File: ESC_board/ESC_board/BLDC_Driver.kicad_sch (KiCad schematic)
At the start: 55 parts, among them IC2 DRV8320, J5 Conn_01x03, Q1 TPH2R306NH1,LQ, Q2 TPH2R306NH1,LQ, Q3 TPH2R306NH1,LQ, Q4 TPH2R306NH1,LQ, Q5 TPH2R306NH1,LQ, Q6 TPH2R306NH1,LQ, U2 INA240A1D, U3 INA240A1D, U4 INA240A1D

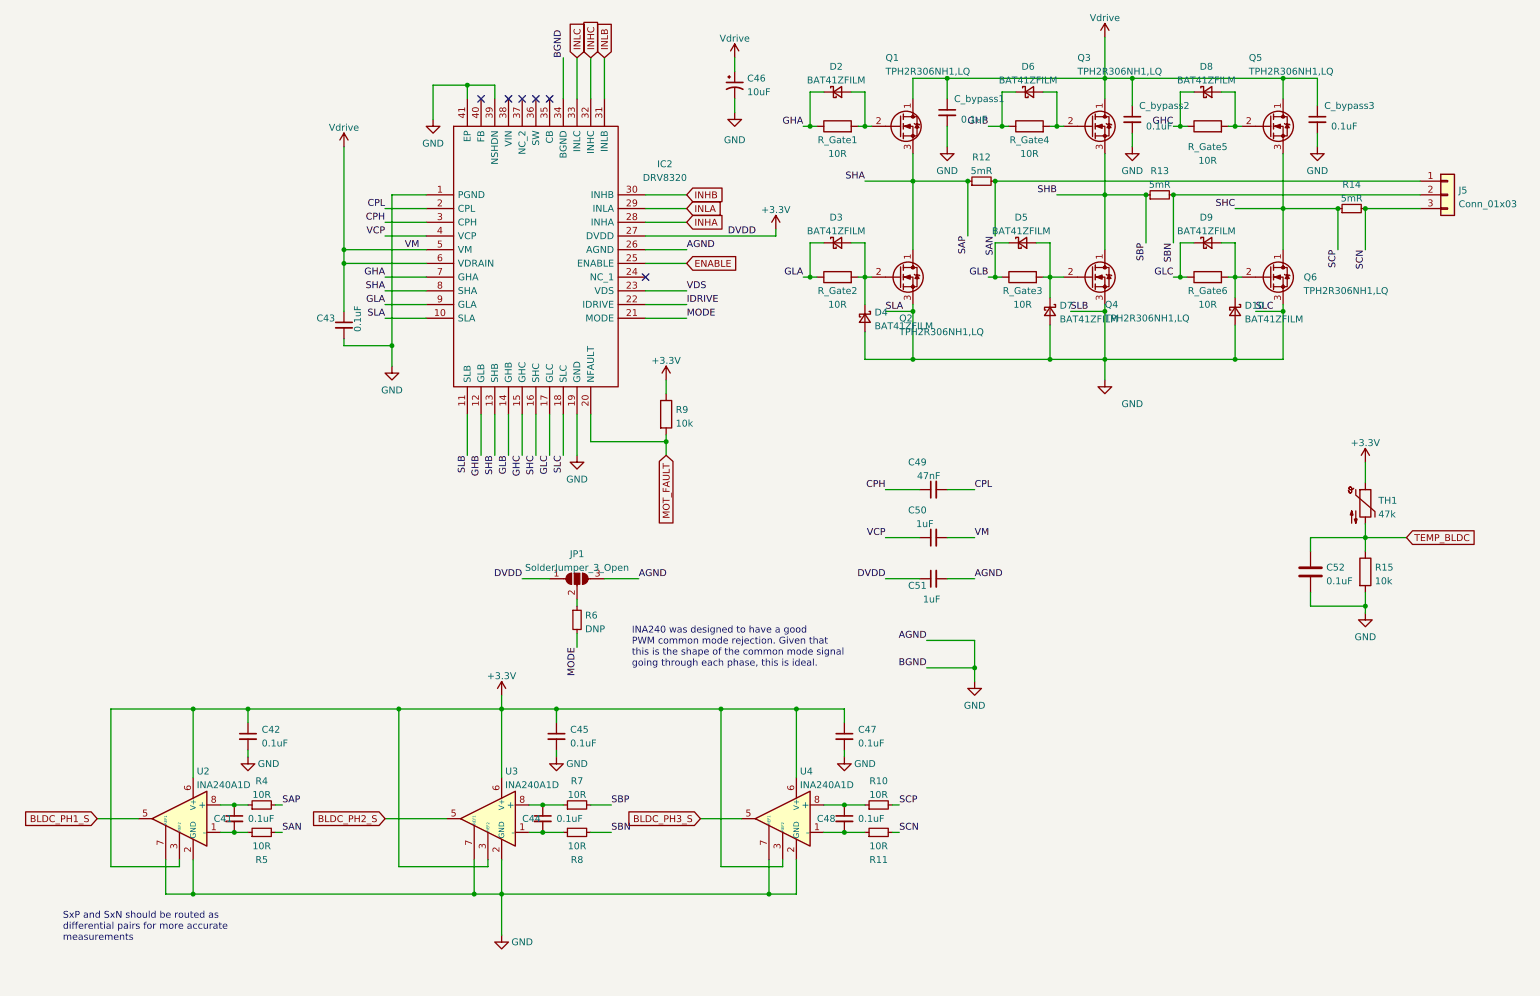
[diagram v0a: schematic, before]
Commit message: Rev 1.2 - Ready for review
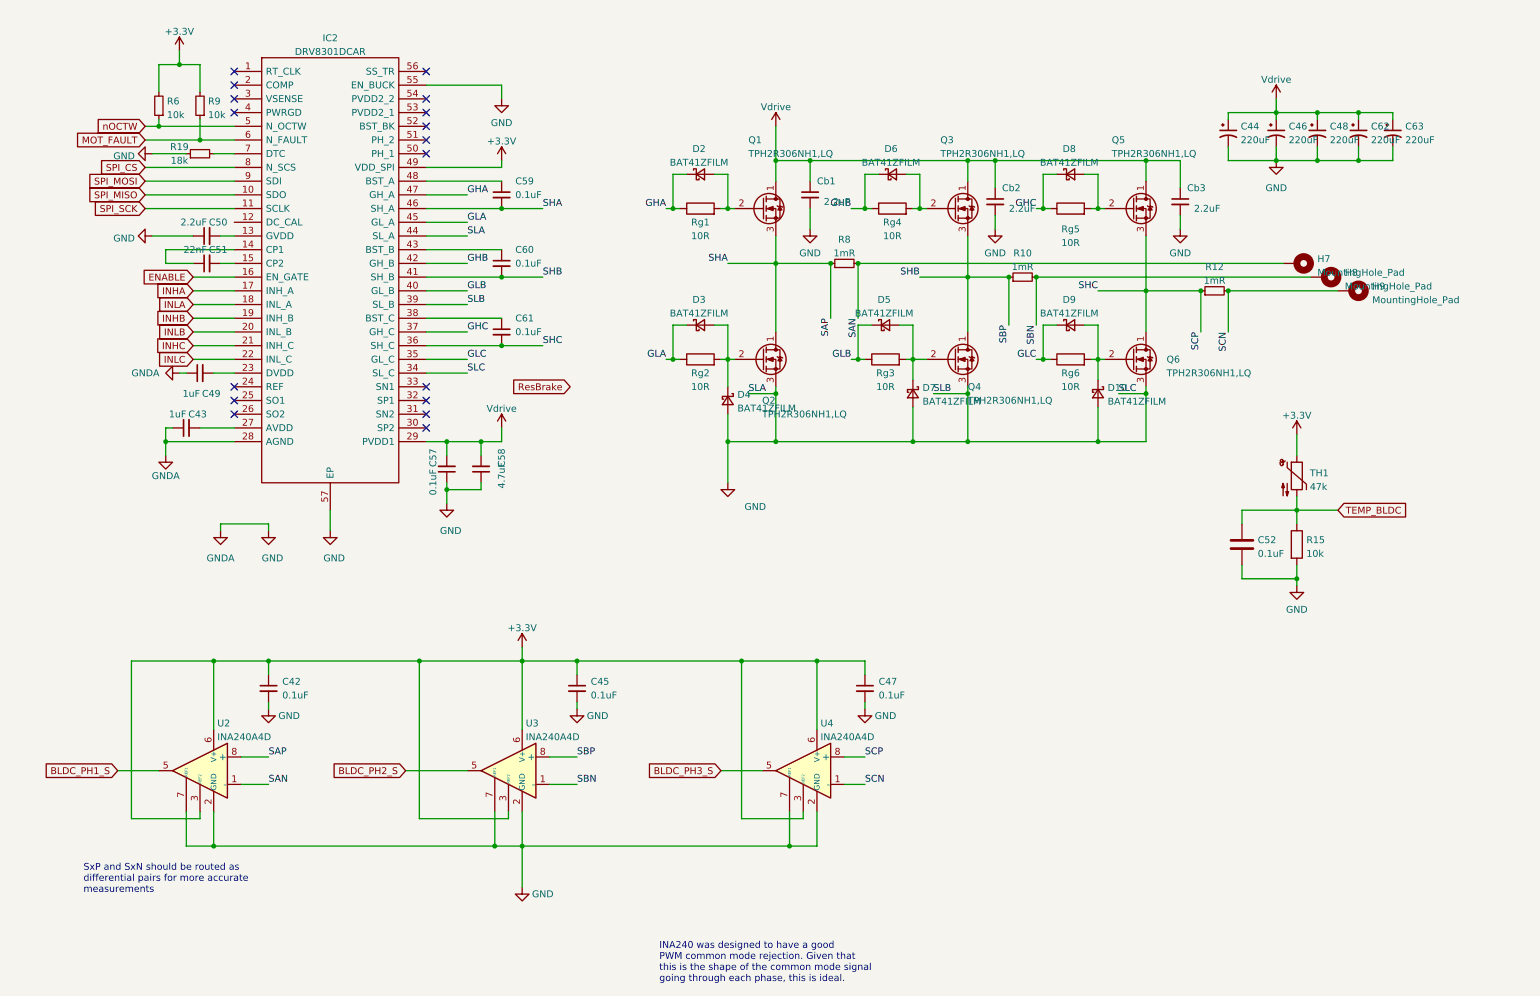
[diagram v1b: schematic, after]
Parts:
- removed C41, C44, C48: 0.1uF, Capacitor_SMD:C_0402_1005Metric_Pad0.74x0.62mm_HandSolder, symbol Device:C_Small
- removed IC2: DRV8320, Package_DFN_QFN:Texas_S-PVQFN-N40_EP4.15x4.15mm_ThermalVias, symbol custom_lib:DRV8320RHRHAT
- removed J5: Conn_01x03, TerminalBlock:TerminalBlock_Altech_AK300-3_P5.00mm, symbol Connector_Generic:Conn_01x03
- removed JP1: SolderJumper_3_Open, Jumper:SolderJumper-3_P2.0mm_Open_TrianglePad1.0x1.5mm_NumberLabels, symbol Jumper:SolderJumper_3_Open
- removed R11, R4, R5, R7: 10R, Resistor_SMD:R_0402_1005Metric_Pad0.72x0.64mm_HandSolder, symbol Device:R_Small
- removed R13, R14: 5mR, Resistor_SMD:R_2010_5025Metric_Pad1.40x2.65mm_HandSolder, symbol Device:R_Small
- removed R9: 10k, Capacitor_SMD:C_0402_1005Metric_Pad0.74x0.62mm_HandSolder, symbol Device:R
- added C44, C48, C62, C63: 220uF, Capacitor_SMD:CP_Elec_5x5.8, symbol Device:C_Polarized_Small_US
- added C57: 0.1uF, Capacitor_SMD:C_0805_2012Metric_Pad1.18x1.45mm_HandSolder, symbol Device:C_Small
- added C58: 4.7uF, Capacitor_SMD:C_0805_2012Metric_Pad1.18x1.45mm_HandSolder, symbol Device:C_Small
- added C59, C60, C61: 0.1uF, Capacitor_SMD:C_0402_1005Metric_Pad0.74x0.62mm_HandSolder, symbol Device:C_Small
- added H7, H8, H9: MountingHole_Pad, Connector_Wire:SolderWire-1.5sqmm_1x01_D1.7mm_OD3.9mm, symbol Mechanical:MountingHole_Pad
- added IC2: DRV8301DCAR, Package_SO:HTSSOP-56-1EP_6.1x14mm_P0.5mm_EP3.61x6.35mm, symbol custom_lib:DRV8301DCAR
- added R19: 18k, Resistor_SMD:R_0402_1005Metric_Pad0.72x0.64mm_HandSolder, symbol Device:R_Small
- added R9: 10k, Resistor_SMD:R_0402_1005Metric_Pad0.72x0.64mm_HandSolder, symbol Device:R_Small
- C43: value 0.1uF -> 1uF
- C46: value 10uF -> 220uF
- C49: value 47nF -> 1uF; footprint Capacitor_SMD:C_0603_1608Metric_Pad1.08x0.95mm_HandSolder -> Capacitor_SMD:C_0402_1005Metric_Pad0.74x0.62mm_HandSolder; Voltage 48V -> 60V
- C50: value 1uF -> 2.2uF; footprint Capacitor_SMD:C_0805_2012Metric_Pad1.18x1.45mm_HandSolder -> Capacitor_SMD:C_0402_1005Metric_Pad0.74x0.62mm_HandSolder; Voltage 16V -> 60V
- C51: value 1uF -> 22nF; footprint Capacitor_SMD:C_0805_2012Metric_Pad1.18x1.45mm_HandSolder -> Capacitor_SMD:C_0603_1608Metric_Pad1.08x0.95mm_HandSolder; Voltage 6.3V -> 100V
- Cb1: renamed from C_bypass1; value 0.1uF -> 2.2uF
- Cb2: renamed from C_bypass2; value 0.1uF -> 2.2uF
- Cb3: renamed from C_bypass3; value 0.1uF -> 2.2uF
- R10, R8: value 10R -> 1mR; footprint Resistor_SMD:R_0402_1005Metric_Pad0.72x0.64mm_HandSolder -> Resistor_SMD:R_2512_6332Metric_Pad1.40x3.35mm_HandSolder; ID (none) -> CSRL3-0R001F8
- R12: value 5mR -> 1mR; footprint Resistor_SMD:R_2010_5025Metric_Pad1.40x2.65mm_HandSolder -> Resistor_SMD:R_2512_6332Metric_Pad1.40x3.35mm_HandSolder; ID TLR2HWDTE5L00F75 -> CSRL3-0R001F8
- R6: value DNP -> 10k
- U2, U3, U4: value INA240A1D -> INA240A4D
- renumbered R_Gate1 to Rg1, R_Gate2 to Rg2, R_Gate3 to Rg3, R_Gate4 to Rg4, R_Gate5 to Rg5, R_Gate6 to Rg6
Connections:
- net CPH is gone; now on net GND: C49.1
- net MODE is gone; now on net +3V3: R6.2
- net VCP is gone; now on net GND: C50.1
- net +3V3: now also IC2.49 (VDD_SPI), R9.2; no longer C51.1
- net ENABLE: now also IC2.16 (EN_GATE)
- net GHA: now also IC2.47 (GH_A)
- net GHB: now also IC2.42 (GH_B)
- net GHC: now also IC2.37 (GH_C)
- net GLA: now also IC2.45 (GL_A)
- net GLB: now also IC2.40 (GL_B)
- net GLC: now also IC2.35 (GL_C)
- net GND: now also C43.1, C44.2, C48.2, C57.1, C58.1, C62.2, C63.2, IC2.28 (AGND), IC2.34 (SL_C), IC2.39 (SL_B), IC2.44 (SL_A), IC2.55 (EN_BUCK), IC2.57 (EP), R19.1; no longer C43.2, C51.2
- net INHA: now also IC2.17 (INH_A)
- net INHB: now also IC2.19 (INH_B)
- net INHC: now also IC2.21 (INH_C)
- net INLA: now also IC2.18 (INL_A)
- net INLB: now also IC2.20 (INL_B)
- net INLC: now also IC2.22 (INL_C)
- net MOT_FAULT: now also IC2.6 (N_FAULT), R9.1
- net SAN: now also R8.2, U2.1 (-), H7.1; no longer R12.2
- net SAP: now also R8.1, U2.8 (+), C59.2, IC2.46 (SH_A); no longer R12.1
- net SBN: now also R10.2, U3.1 (-), H8.1; no longer R8.2
- net SBP: now also R10.1, U3.8 (+), C60.2, IC2.41 (SH_B)
- net SCN: now also R12.2, U4.1 (-), H9.1
- net SCP: now also R12.1, U4.8 (+), C61.2, IC2.36 (SH_C); no longer R10.2
- net Vdrive: now also C44.1, C48.1, C57.2, C58.2, C62.1, C63.1, IC2.29 (PVDD1); no longer C43.1, C50.2
- net nOCTW: now reaches R6.1
- net nOCTW: now also IC2.5 (N_OCTW)
- net CPL: no longer names the net of C49.2
- net CPL: now also IC2.23 (DVDD)
- new net: IC2.7 (DTC), R19.2
- new net: C43.2, IC2.27 (AVDD)
- new net: C61.1, IC2.38 (BST_C)
- new net: C60.1, IC2.43 (BST_B)
- new net: C50.2, IC2.13 (GVDD)
- new net: C59.1, IC2.48 (BST_A)
- new net: C51.1, IC2.14 (CP1)
- new net: C51.2, IC2.15 (CP2)
- new net SPI_CS: IC2.8 (N_SCS)
- new net SPI_MISO: IC2.10 (SDO)
- new net SPI_MOSI: IC2.9 (SDI)
- new net SPI_SCK: IC2.11 (SCLK)
- no-connect marks 6 -> 17
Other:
- moved on the sheet: C42, C45, C46, C47, C52, Cb1, Cb2, Cb3, D10, D2, D3, D4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
